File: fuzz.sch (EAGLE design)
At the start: 19 parts, among them T1 2N3904, T2 2N3904

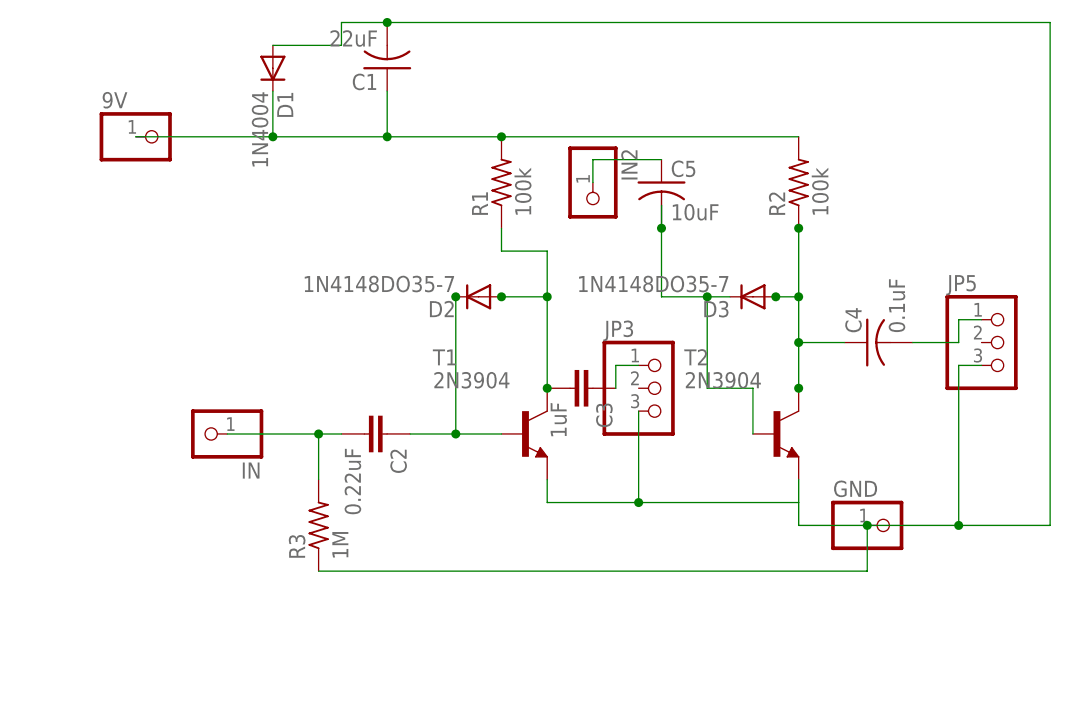
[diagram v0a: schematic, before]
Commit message: 1.1
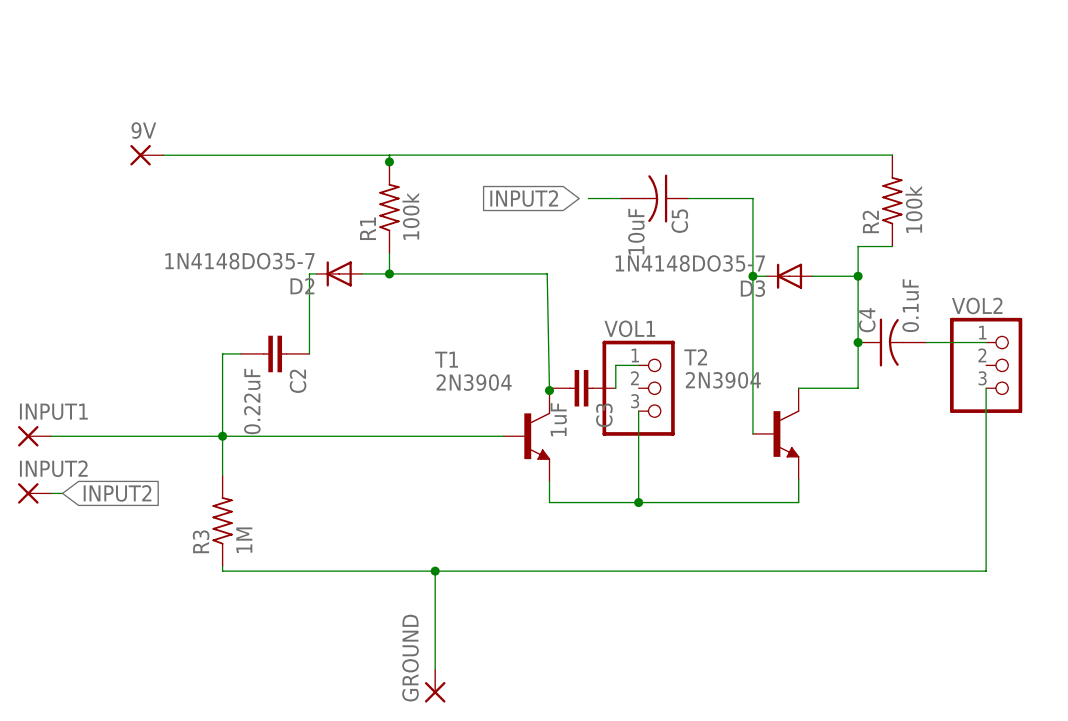
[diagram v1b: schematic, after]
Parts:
- removed C1: 22uF, resistor:C-US025-024X044
- removed D1: 1N4004, diode:1N4004
- removed GND, IN, IN2: (no value), pinhead:PINHD-1X1
- removed JP5: (no value), pinhead:PINHD-1X3
- added GROUND, INPUT1, INPUT2: (no value), wirepad:2,15/1,0
- added VOL2: (no value), pinhead:PINHD-1X3
- 9V: device pinhead:PINHD-1X1 -> wirepad:2,15/1,0
- renumbered JP3 to VOL1
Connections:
- removed net INPUT: C2.2, IN.1, R3.2
- removed net N$7: C5.1, IN2.1
- new net INPUT2: C5.2, INPUT2.P
- new net N$10: GROUND.P, R3.1, VOL2.3
- new net N$11: C2.1, D2.C
- net N$2: now also C2.2, INPUT1.P, R3.2; no longer C2.1, D2.C
- net N$4: now also C5.1, D3.C, T2.B; no longer 9V.1, C1.1, D1.C, R1.2, R2.2
- net N$6: now also 9V.P, R1.2, R2.2; no longer C5.2, D3.C, T2.B
- net N$8: now also VOL2.1; no longer JP5.1
- net N$9: no longer C1.2, D1.A, GND.1, JP5.3, R3.1
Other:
- moved on the sheet: C2, C4, C5, D2, D3, R1, R2, R3
